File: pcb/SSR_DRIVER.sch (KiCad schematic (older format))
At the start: 14 parts, among them Q1 2N3904(1AM), U2 OMRON-G3MB-202P

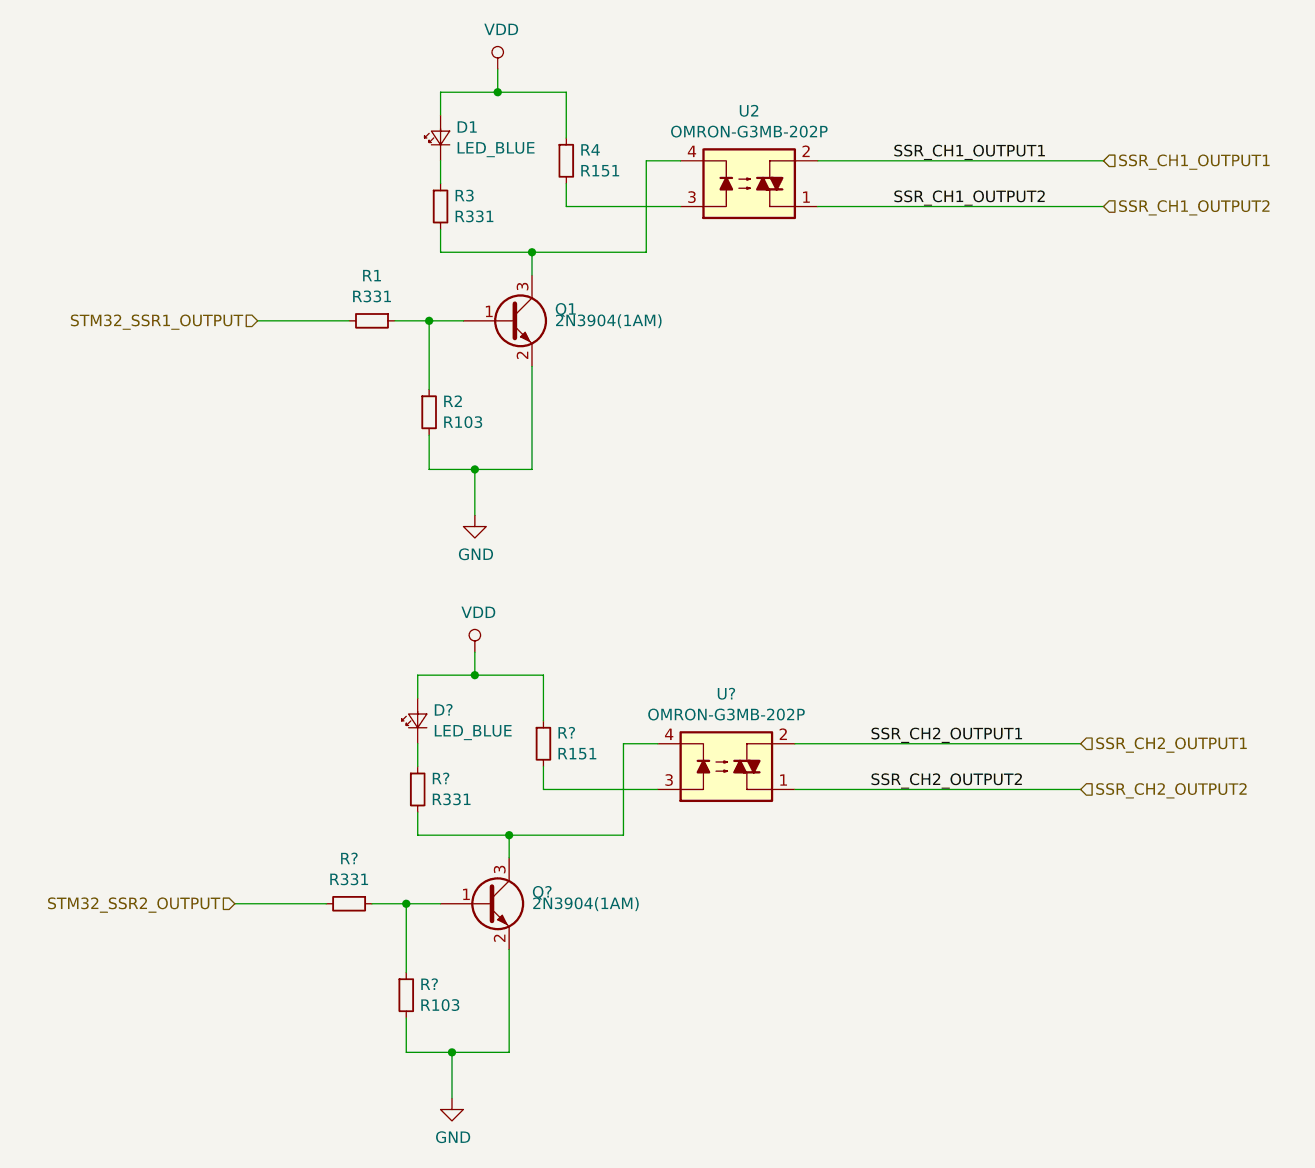
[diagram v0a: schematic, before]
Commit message: update,
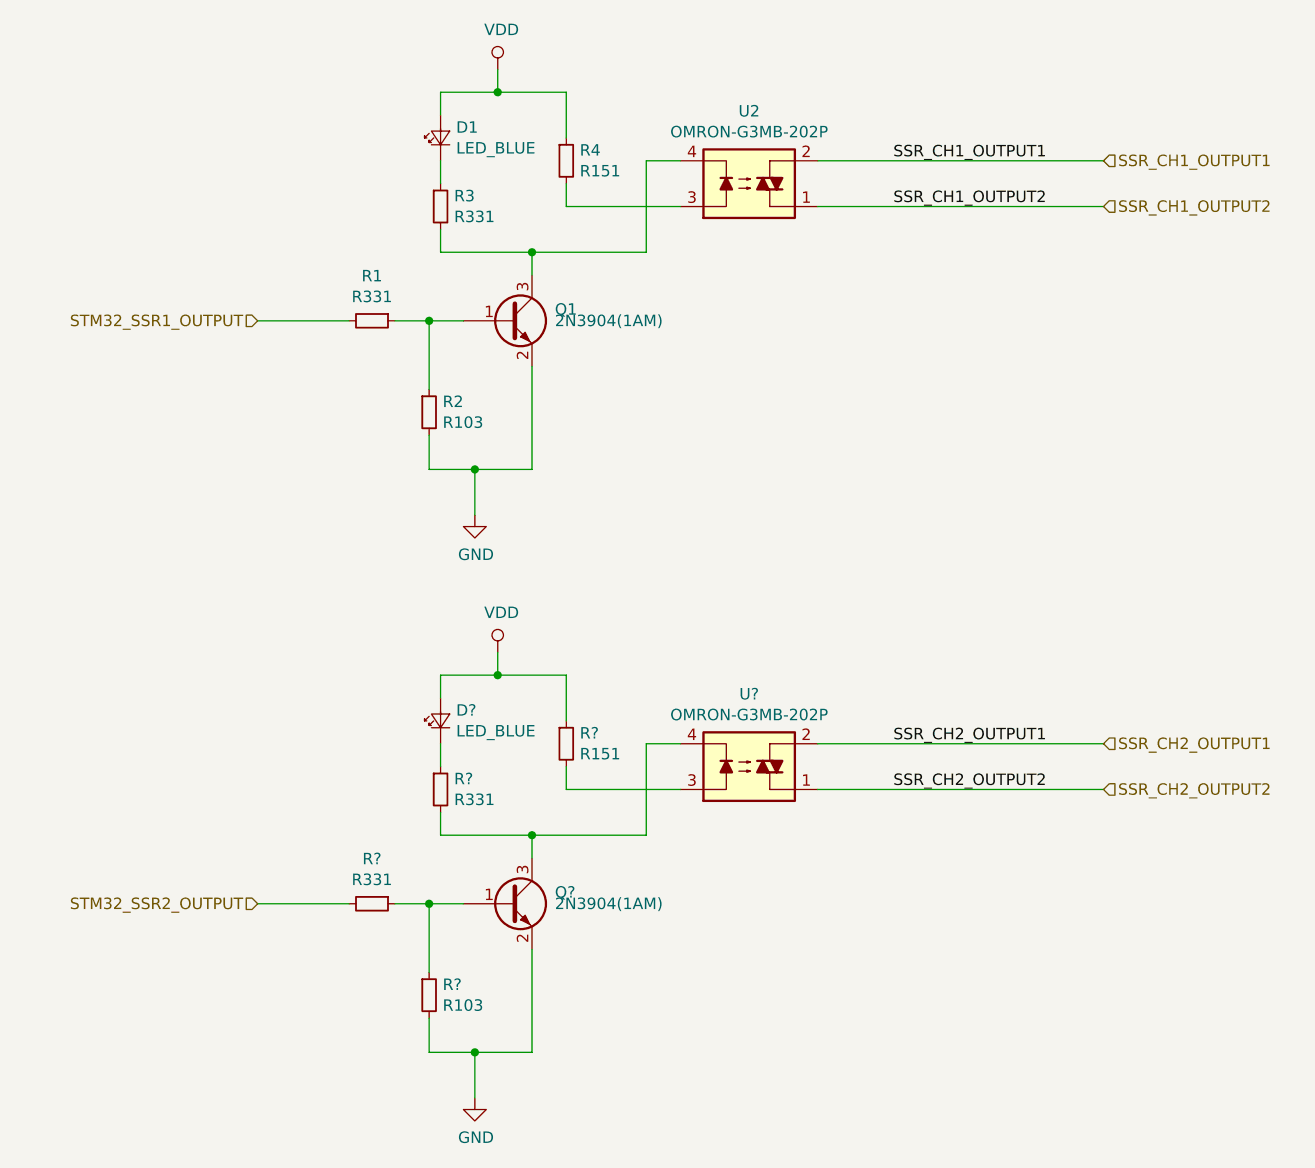
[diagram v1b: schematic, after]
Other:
- moved on the sheet: D?, Q?, R?, U?
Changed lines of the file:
@@
 L taobao-r:R331 R?
 U 1 1 5BE460BB
-P 4400 5550
+P 4500 5550
 AR Path="/5BCB4A39/5BE460BB" Ref="R?"  Part="1"
 AR Path="/5BE41138/5BE460BB" Ref="R?"  Part="1"
-F 0 "R?" V 4204 5550 50  0000 C CNN
-F 1 "R331" V 4295 5550 50  0000 C CNN
-F 2 "Resistor_SMD:R_0805_2012Metric_Pad1.15x1.40mm_HandSolder" H 4400 5550 50  0001 C CNN
-F 3 "~" H 4400 5550 50  0001 C CNN
-	1    4400 5550
+F 0 "R?" V 4304 5550 50  0000 C CNN
+F 1 "R331" V 4395 5550 50  0000 C CNN
+F 2 "Resistor_SMD:R_0805_2012Metric_Pad1.15x1.40mm_HandSolder" H 4500 5550 50  0001 C CNN
+F 3 "~" H 4500 5550 50  0001 C CNN
+	1    4500 5550
 	0    1    1    0
 $EndComp
-Text HLabel 3900 5550 0    50   Input ~ 0
+Text HLabel 4000 5550 0    50   Input ~ 0
 STM32_SSR2_OUTPUT
 $Comp
 L taobao-r:R103 R?
 U 1 1 5BE460C2
-P 4650 5950
+P 4750 5950
 AR Path="/5BCB4A39/5BE460C2" Ref="R?"  Part="1"
 AR Path="/5BE41138/5BE460C2" Ref="R?"  Part="1"
-F 0 "R?" H 4709 5996 50  0000 L CNN
-F 1 "R103" H 4709 5905 50  0000 L CNN
-F 2 "Resistor_SMD:R_0805_2012Metric_Pad1.15x1.40mm_HandSolder" H 4650 5950 50  0001 C CNN
-F 3 "~" H 4650 5950 50  0001 C CNN
-	1    4650 5950
+F 0 "R?" H 4809 5996 50  0000 L CNN
+F 1 "R103" H 4809 5905 50  0000 L CNN
+F 2 "Resistor_SMD:R_0805_2012Metric_Pad1.15x1.40mm_HandSolder" H 4750 5950 50  0001 C CNN
+F 3 "~" H 4750 5950 50  0001 C CNN
+	1    4750 5950
 	1    0    0    -1
 $EndComp
 Wire Wire Line
-	3900 5550 4300 5550
+	4000 5550 4400 5550
 Wire Wire Line
-	4500 5550 4650 5550
+	4600 5550 4750 5550
 Wire Wire Line
-	4650 5550 4650 5850
+	4750 5550 4750 5850
 Wire Wire Line
-	4800 5550 4650 5550
-Connection ~ 4650 5550
+	4900 5550 4750 5550
+Connection ~ 4750 5550
 Wire Wire Line
-	4650 6050 4650 6200
+	4750 6050 4750 6200
 Wire Wire Line
-	4650 6200 4850 6200
+	4750 6200 4950 6200
 Wire Wire Line
-	5100 6200 5100 5750
+	5200 6200 5200 5750
 $Comp
 L power:GND #PWR?
 U 1 1 5BE460D0
-P 4850 6400
+P 4950 6400
 AR Path="/5BCB4A39/5BE460D0" Ref="#PWR?"  Part="1"
 AR Path="/5BE41138/5BE460D0" Ref="#PWR?"  Part="1"
-F 0 "#PWR?" H 4850 6150 50  0001 C CNN
-F 1 "GND" H 4855 6227 50  0000 C CNN
-F 2 "" H 4850 6400 50  0001 C CNN
-F 3 "" H 4850 6400 50  0001 C CNN
-	1    4850 6400
+F 0 "#PWR?" H 4950 6150 50  0001 C CNN
+F 1 "GND" H 4955 6227 50  0000 C CNN
+F 2 "" H 4950 6400 50  0001 C CNN
+F 3 "" H 4950 6400 50  0001 C CNN
+	1    4950 6400
 	1    0    0    -1
 $EndComp
 Wire Wire Line
-	4850 6400 4850 6200
-Connection ~ 4850 6200
+	4950 6400 4950 6200
+Connection ~ 4950 6200
 Wire Wire Line
-	4850 6200 5100 6200
+	4950 6200 5200 6200
 $Comp
 L taobao-components:LED_RED D?
 U 1 1 5BE460D9
-P 4700 4750
+P 4800 4750
 AR Path="/5BCB4A39/5BE460D9" Ref="D?"  Part="1"
 AR Path="/5BE41138/5BE460D9" Ref="D?"  Part="1"
-F 0 "D?" V 4746 4682 50  0000 R CNN
-F 1 "LED_BLUE" V 4655 4682 50  0000 R CNN
-F 2 "LED_SMD:LED_0805_2012Metric_Pad1.15x1.40mm_HandSolder" V 4700 4750 50  0001 C CNN
-F 3 "~" V 4700 4750 50  0001 C CNN
-	1    4700 4750
+F 0 "D?" V 4846 4682 50  0000 R CNN
+F 1 "LED_BLUE" V 4755 4682 50  0000 R CNN
+F 2 "LED_SMD:LED_0805_2012Metric_Pad1.15x1.40mm_HandSolder" V 4800 4750 50  0001 C CNN
+F 3 "~" V 4800 4750 50  0001 C CNN
+	1    4800 4750
 	0    -1   -1   0
 $EndComp
@@
 L taobao-r:R331 R?
 U 1 1 5BE460DF
-P 4700 5050
+P 4800 5050
 AR Path="/5BCB4A39/5BE460DF" Ref="R?"  Part="1"
 AR Path="/5BE41138/5BE460DF" Ref="R?"  Part="1"
-F 0 "R?" H 4759 5096 50  0000 L CNN
-F 1 "R331" H 4759 5005 50  0000 L CNN
-F 2 "Resistor_SMD:R_0805_2012Metric_Pad1.15x1.40mm_HandSolder" H 4700 5050 50  0001 C CNN
-F 3 "~" H 4700 5050 50  0001 C CNN
-	1    4700 5050
+F 0 "R?" H 4859 5096 50  0000 L CNN
+F 1 "R331" H 4859 5005 50  0000 L CNN
+F 2 "Resistor_SMD:R_0805_2012Metric_Pad1.15x1.40mm_HandSolder" H 4800 5050 50  0001 C CNN
+F 3 "~" H 4800 5050 50  0001 C CNN
+	1    4800 5050
 	1    0    0    -1
 $EndComp
 Wire Wire Line
-	4700 5150 4700 5250
+	4800 5150 4800 5250
 Wire Wire Line
-	4700 5250 5100 5250
+	4800 5250 5200 5250
 Wire Wire Line
-	5100 5250 5100 5350
+	5200 5250 5200 5350
 Wire Wire Line
-	4700 4550 4700 4650
+	4800 4550 4800 4650
 Wire Wire Line
-	4700 4850 4700 4950
+	4800 4850 4800 4950
 $Comp
 L taobao-r:R151 R?
 U 1 1 5BE460EA
-P 5250 4850
+P 5350 4850
 AR Path="/5BCB4A39/5BE460EA" Ref="R?"  Part="1"
 AR Path="/5BE41138/5BE460EA" Ref="R?"  Part="1"
-F 0 "R?" H 5309 4896 50  0000 L CNN
-F 1 "R151" H 5309 4805 50  0000 L CNN
-F 2 "Resistor_SMD:R_0805_2012Metric_Pad1.15x1.40mm_HandSolder" H 5250 4850 50  0001 C CNN
-F 3 "~" H 5250 4850 50  0001 C CNN
-	1    5250 4850
+F 0 "R?" H 5409 4896 50  0000 L CNN
+F 1 "R151" H 5409 4805 50  0000 L CNN
+F 2 "Resistor_SMD:R_0805_2012Metric_Pad1.15x1.40mm_HandSolder" H 5350 4850 50  0001 C CNN
+F 3 "~" H 5350 4850 50  0001 C CNN
+	1    5350 4850
 	1    0    0    -1
 $EndComp
 Wire Wire Line
-	5250 4550 5250 4750
+	5350 4550 5350 4750
 $Comp
 L Relay_SolidState:S102S01 U?
 U 1 1 5BE460F1
-P 6050 4950
+P 6150 4950
 AR Path="/5BCB4A39/5BE460F1" Ref="U?"  Part="1"
 AR Path="/5BE41138/5BE460F1" Ref="U?"  Part="1"
-F 0 "U?" H 6050 4633 50  0000 C CNN
-F 1 "OMRON-G3MB-202P" H 6050 4724 50  0000 C CNN
-F 2 "footprint-lib:OMRON-G3MB-202P" H 5850 4750 50  0001 L CIN
-F 3 "http://www.sharp-world.com/products/device/lineup/data/pdf/datasheet/s102s01_e.pdf" H 6015 4950 50  0001 L CNN
-	1    6050 4950
+F 0 "U?" H 6150 4633 50  0000 C CNN
+F 1 "OMRON-G3MB-202P" H 6150 4724 50  0000 C CNN
+F 2 "footprint-lib:OMRON-G3MB-202P" H 5950 4750 50  0001 L CIN
+F 3 "http://www.sharp-world.com/products/device/lineup/data/pdf/datasheet/s102s01_e.pdf" H 6115 4950 50  0001 L CNN
+	1    6150 4950
 	1    0    0    1
 $EndComp
 Wire Wire Line
-	5250 4950 5250 5050
+	5350 4950 5350 5050
 Wire Wire Line
-	5250 5050 5750 5050
+	5350 5050 5850 5050
 Wire Wire Line
-	5100 5250 5600 5250
+	5200 5250 5700 5250
 Wire Wire Line
-	5600 5250 5600 4850
+	5700 5250 5700 4850
 Wire Wire Line
-	5600 4850 5750 4850
-Connection ~ 5100 5250
-Text Label 7350 4850 2    50   ~ 0
+	5700 4850 5850 4850
+Connection ~ 5200 5250
+Text Label 7450 4850 2    50   ~ 0
 SSR_CH2_OUTPUT1
-Text Label 7350 5050 2    50   ~ 0
+Text Label 7450 5050 2    50   ~ 0
 SSR_CH2_OUTPUT2
-Text HLabel 7600 4850 2    50   Input ~ 0
+Text HLabel 7700 4850 2    50   Input ~ 0
 SSR_CH2_OUTPUT1
-Text HLabel 7600 5050 2    50   Input ~ 0
+Text HLabel 7700 5050 2    50   Input ~ 0
 SSR_CH2_OUTPUT2
 Wire Wire Line
-	6350 4850 7600 4850
+	6450 4850 7700 4850
 Wire Wire Line
-	6350 5050 7600 5050
+	6450 5050 7700 5050
 $Comp
 L power:VDD #PWR?
 U 1 1 5BE46103
-P 4950 4450
+P 5050 4450
 AR Path="/5BCB4A39/5BE46103" Ref="#PWR?"  Part="1"
 AR Path="/5BE41138/5BE46103" Ref="#PWR?"  Part="1"
-F 0 "#PWR?" H 4950 4300 50  0001 C CNN
-F 1 "VDD" H 4967 4623 50  0000 C CNN
-F 2 "" H 4950 4450 50  0001 C CNN
-F 3 "" H 4950 4450 50  0001 C CNN
-	1    4950 4450
+F 0 "#PWR?" H 5050 4300 50  0001 C CNN
+F 1 "VDD" H 5067 4623 50  0000 C CNN
+F 2 "" H 5050 4450 50  0001 C CNN
+F 3 "" H 5050 4450 50  0001 C CNN
+	1    5050 4450
 	1    0    0    -1
 $EndComp
 Wire Wire Line
-	4950 4450 4950 4550
+	5050 4450 5050 4550
 Wire Wire Line
-	4950 4550 4700 4550
+	5050 4550 4800 4550
 Wire Wire Line
-	4950 4550 5250 4550
-Connection ~ 4950 4550
+	5050 4550 5350 4550
+Connection ~ 5050 4550
 $Comp
 L taobao-transistor:2N3904(1AM) Q?
 U 1 1 5BE4610D
-P 5000 5550
+P 5100 5550
 AR Path="/5BE4610D" Ref="Q?"  Part="1"
 AR Path="/5BCB4A39/5BE4610D" Ref="Q?"  Part="1"
 AR Path="/5BE41138/5BE4610D" Ref="Q?"  Part="1"
-F 0 "Q?" H 5200 5600 50  0000 L CNN
-F 1 "2N3904(1AM)" H 5200 5550 50  0000 L CNN
-F 2 "Package_TO_SOT_SMD:SOT-23_Handsoldering" H 5200 5475 50  0001 L CIN
-F 3 "" H 5000 5550 50  0001 L CNN
-	1    5000 5550
+F 0 "Q?" H 5300 5600 50  0000 L CNN
+F 1 "2N3904(1AM)" H 5300 5550 50  0000 L CNN
+F 2 "Package_TO_SOT_SMD:SOT-23_Handsoldering" H 5300 5475 50  0001 L CIN
+F 3 "" H 5100 5550 50  0001 L CNN
+	1    5100 5550
 	1    0    0    -1
 $EndComp
